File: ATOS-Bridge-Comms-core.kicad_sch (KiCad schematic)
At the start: 61 parts, among them J2 Conn_02x05_Counter_Clockwise, J3 Conn_01x09_Pin, Q1 2SC4617R, Q3 UMH3N, SW2 SKRPACE010, SW3 SKRPACE010, U1 LAN8720A-CP-TR, U2 AMS1117-3.3, U3 CH340C, U4 ESP32-WROOM-32UE, X1 ECS-2520MV-250-CN-TR

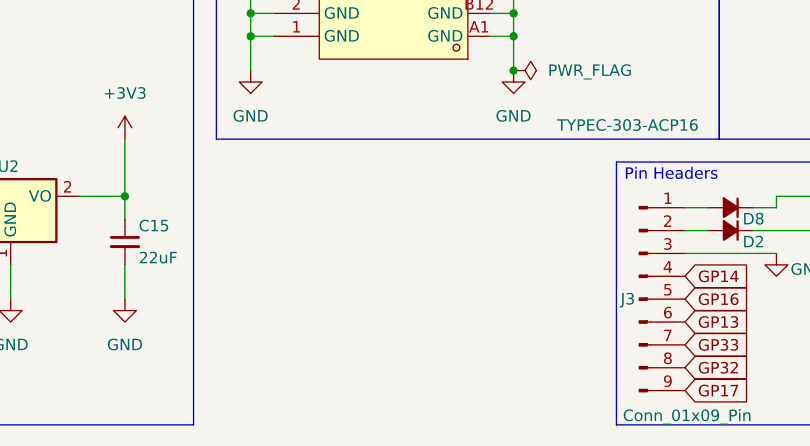
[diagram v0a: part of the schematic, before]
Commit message: Post-design review interim changes
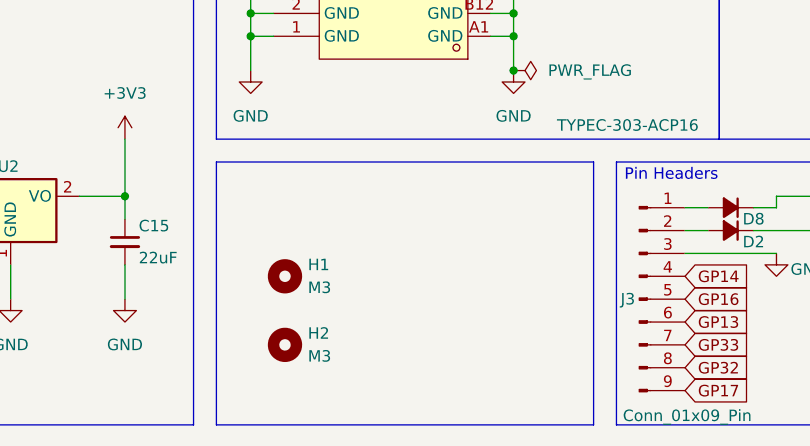
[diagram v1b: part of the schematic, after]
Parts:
- added H1, H2: M3, MountingHole:MountingHole_3.2mm_M3, symbol Mechanical:MountingHole
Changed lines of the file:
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@@
 	)
 	(rectangle
+		(start 55.88 166.37)
+		(end 97.79 195.58)
+		(stroke
+			(width 0)
+			(type default)
+		)
+		(fill
+			(type none)
+		)
+	)
+	(rectangle
 		(start 55.88 97.79)
 		(end 111.76 163.83)
@@
 	)
 	(symbol
+		(lib_id "Mechanical:MountingHole")
+		(at 63.5 186.69 0)
+		(unit 1)
+		(body_style 1)
+		(exclude_from_sim no)
+		(in_bom no)
+		(on_board yes)
+		(in_pos_files yes)
+		(dnp no)
+		(fields_autoplaced yes)
+		(property "Reference" "H2"
+			(at 66.04 185.4199 0)
+			(show_name no)
+			(do_not_autoplace no)
+			(effects
+				(font
+					(size 1.27 1.27)
+				)
+				(justify left)
+			)
+		)
+		(property "Value" "M3"
+			(at 66.04 187.9599 0)
+			(show_name no)
+			(do_not_autoplace no)
+			(effects
+				(font
+					(size 1.27 1.27)
+				)
+				(justify left)
+			)
+		)
+		(property "Footprint" "MountingHole:MountingHole_3.2mm_M3"
+			(at 63.5 186.69 0)
+			(hide yes)
+			(show_name no)
+			(do_not_autoplace no)
+			(effects
+				(font
+					(size 1.27 1.27)
+				)
+			)
+		)
+		(property "Datasheet" ""
+			(at 63.5 186.69 0)
+			(hide yes)
+			(show_name no)
+			(do_not_autoplace no)
+			(effects
+				(font
+					(size 1.27 1.27)
+				)
+			)
+		)
+		(property "Description" "Mounting Hole without connection"
+			(at 63.5 186.69 0)
+			(hide yes)
+			(show_name no)
+			(do_not_autoplace no)
+			(effects
+				(font
+					(size 1.27 1.27)
+				)
+			)
+		)
+		(instances
+			(project "ATOS-Bridge-Comms-core"
+				(path "/2b46a950-adb6-434b-928c-c069ab58e33e"
+					(reference "H2")
+					(unit 1)
+				)
+			)
+		)
+	)
+	(symbol
 		(lib_id "power:GND")
 		(at 100.33 31.75 0)
@@
 					(unit 1)
 				)
+			)
+		)
+	)
+	(symbol
+		(lib_id "Mechanical:MountingHole")
+		(at 63.5 179.07 0)
+		(unit 1)
+		(body_style 1)
+		(exclude_from_sim no)
+		(in_bom no)
+		(on_board yes)
+		(in_pos_files yes)
+		(dnp no)
+		(fields_autoplaced yes)
+		(property "Reference" "H1"
+			(at 66.04 177.7999 0)
+			(show_name no)
+			(do_not_autoplace no)
+			(effects
+				(font
+					(size 1.27 1.27)
+				)
+				(justify left)
+			)
+		)
+		(property "Value" "M3"
+			(at 66.04 180.3399 0)
+			(show_name no)
+			(do_not_autoplace no)
+			(effects
+				(font
+					(size 1.27 1.27)
+				)
+				(justify left)
+			)
+		)
+		(property "Footprint" "MountingHole:MountingHole_3.2mm_M3"
+			(at 63.5 179.07 0)
+			(hide yes)
+			(show_name no)
+			(do_not_autoplace no)
+			(effects
+				(font
+					(size 1.27 1.27)
+				)
+			)
+		)
+		(property "Datasheet" ""
+			(at 63.5 179.07 0)
+			(hide yes)
+			(show_name no)
+			(do_not_autoplace no)
+			(effects
+				(font
+					(size 1.27 1.27)
+				)
+			)
+		)
+		(property "Description" "Mounting Hole without connection"
+			(at 63.5 179.07 0)
+			(hide yes)
+			(show_name no)
+			(do_not_autoplace no)
+			(effects
+				(font
+					(size 1.27 1.27)
+				)
+			)
+		)
+		(instances
+			(project "ATOS-Bridge-Comms-core"
+				(path "/2b46a950-adb6-434b-928c-c069ab58e33e"
+					(reference "H1")
+					(unit 1)
+				)
